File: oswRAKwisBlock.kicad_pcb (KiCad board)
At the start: 2 copper layers, 33.8 x 46 mm, 33 parts, among them J1 WisBlock, J2 0524352471, J3 USB_B_Micro, J4 10114830-10102LF, Q1 SI1308EDL-T1-GE3, U1 MCP73811T-420I/OT

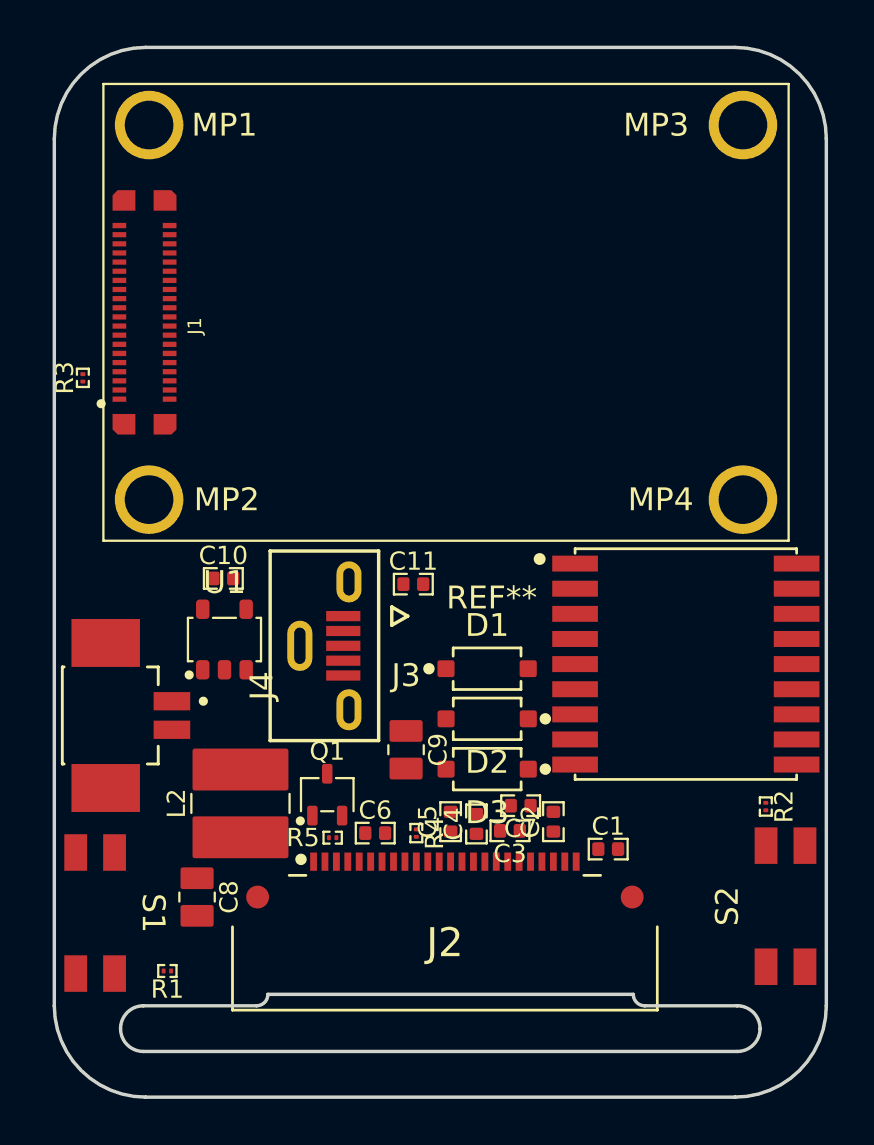
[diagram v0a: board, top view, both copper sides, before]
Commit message: Adding a bunch of stuff to the design and some local models.
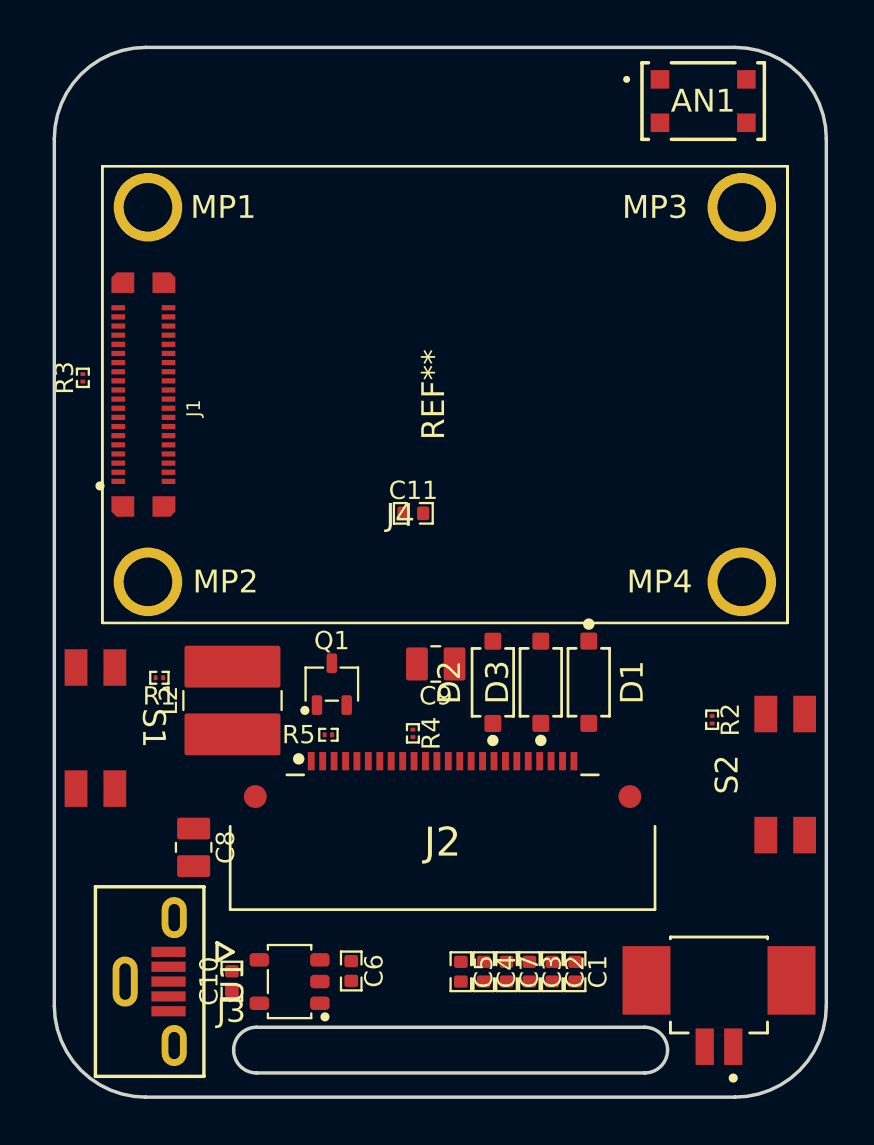
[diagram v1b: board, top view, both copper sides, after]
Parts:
- removed the REF** at (147.5, 127.0)
- added AN1: 1.575GHz ANT, AllardANT:MOLEX_1462350001_CHIP, F.Cu at (148.3, 102.3)
- added REF**: RAK11310, oswRAKlib:RAK11310, F.Cu at (136.9, 115.2)
- added REF**: 1.54 E-Paper Display, oswRAKlib:154_Epaper_Display, B.Cu at (136.8, 122.5)
- moved J4 29.1 mm to (148.9, 141.1), turned to 180 degrees
- moved C10 17.6 mm to (127.6, 140.9), turned to 90 degrees
- moved J3 16.6 mm to (124.0, 140.9)
- moved U1 15.2 mm to (130.2, 140.9), turned to 90 degrees
- moved R1 12.8 mm to (124.5, 127.6)
- moved S1 8.10 mm to (121.7, 129.8)
- moved C7 7.29 mm to (139.7, 140.5), turned to -90 degrees
- moved C5 6.58 mm to (137.7, 140.5), turned to -90 degrees
- moved C2 6.57 mm to (141.7, 140.5), turned to -90 degrees
- moved C4 6.48 mm to (138.7, 140.5), turned to -90 degrees
- moved C3 6.23 mm to (140.7, 140.5), turned to -90 degrees
- moved C6 6.13 mm to (132.8, 140.4), turned to -90 degrees
- moved S2 5.76 mm to (151.8, 131.8)
- moved C1 5.56 mm to (142.7, 140.5), turned to -90 degrees
- moved Q1 4.84 mm to (132.0, 127.9)
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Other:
- outline, holes or cut-outs redrawn
- copper layers 2 -> 4
